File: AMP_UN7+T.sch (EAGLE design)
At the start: 55 parts

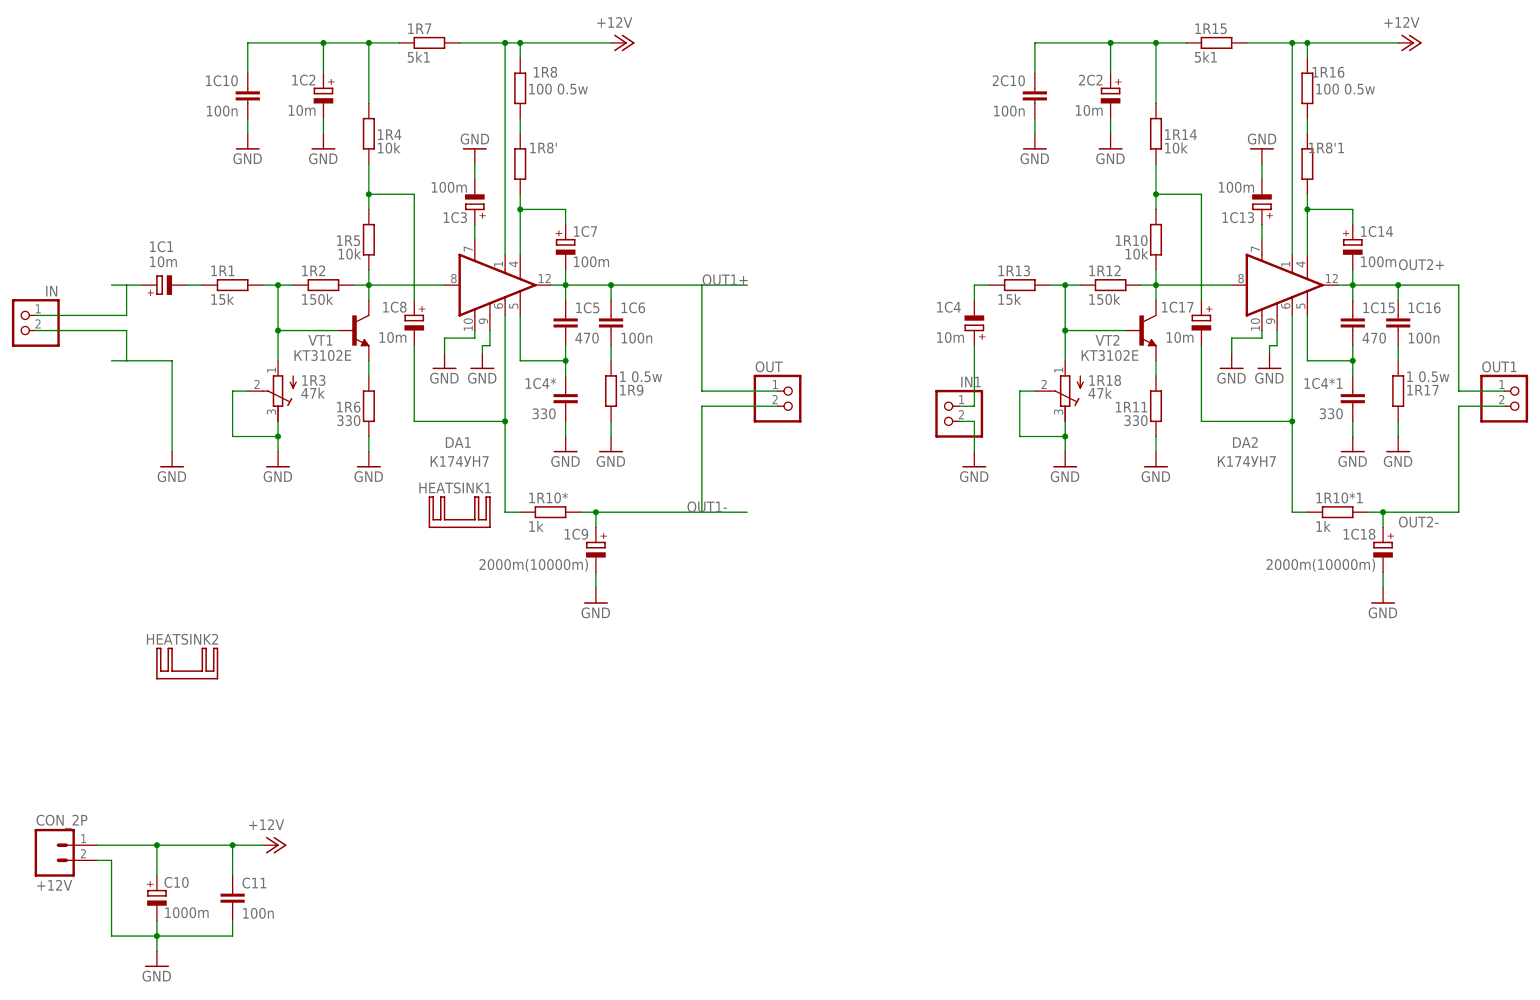
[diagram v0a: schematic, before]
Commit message: 4
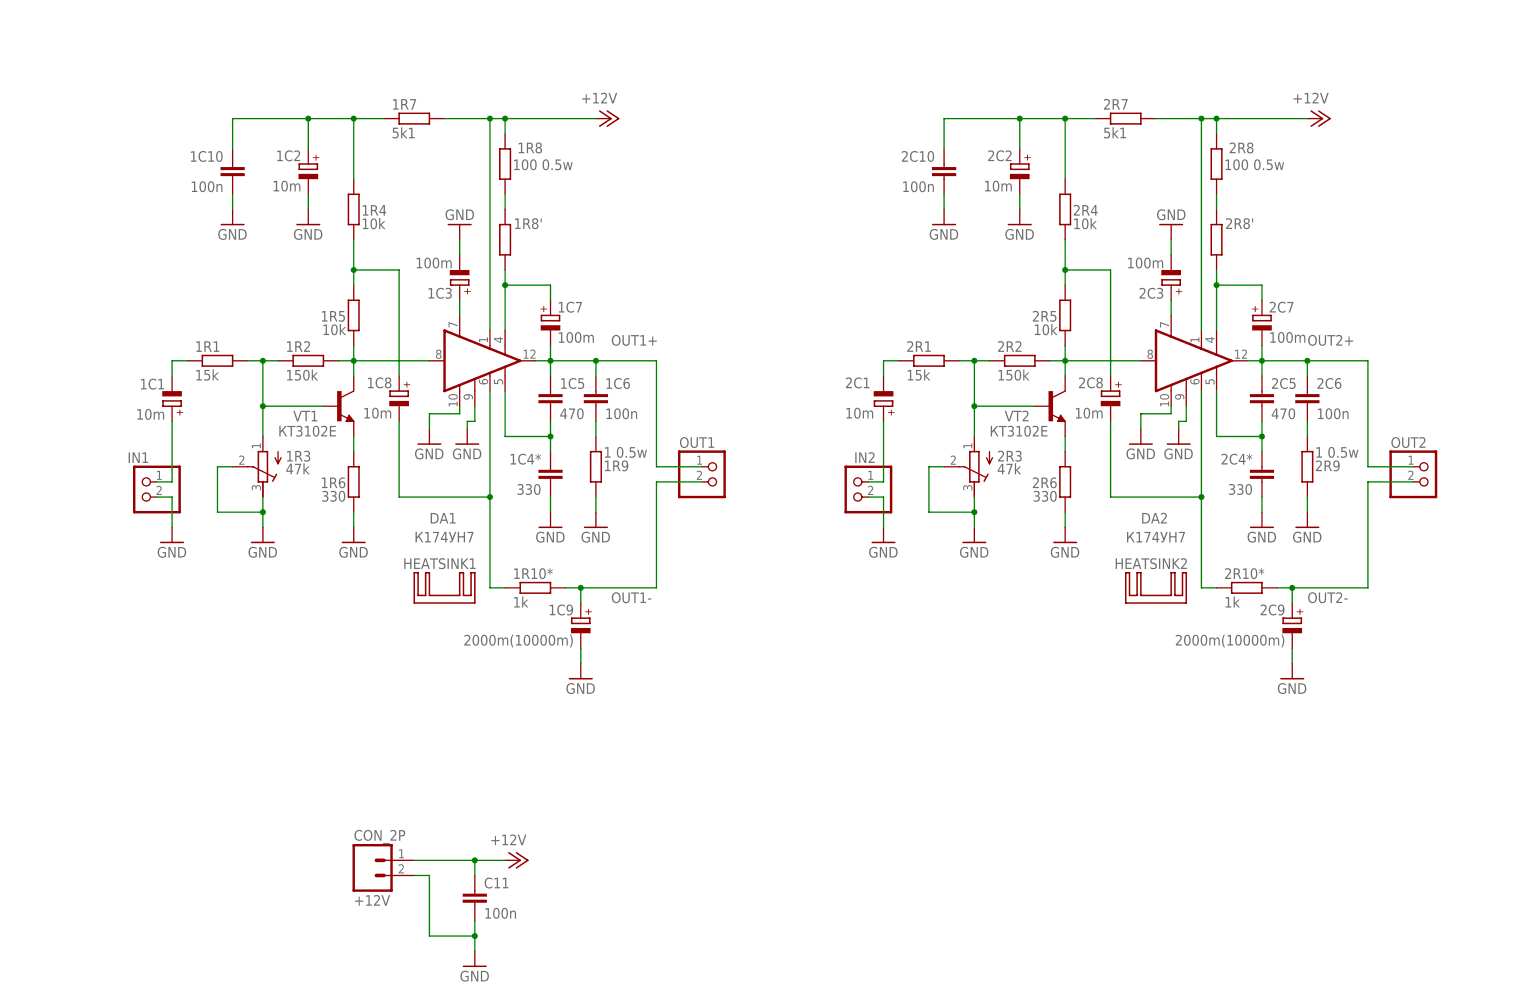
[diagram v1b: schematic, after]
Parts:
- removed 1C13: 100m, rcl:CPOL-EUE2.5-6
- removed 1C14: 100m, rcl:CPOL-EUE2.5-5
- removed 1C15: 470, rcl:C-EU050-030X075
- removed 1C16: 100n, rcl:C-EU075-052X106
- removed 1C17, 1C4: 10m, rcl:CPOL-EUE2.5-5
- removed 1C18: 2000m(10000m), rcl:CPOL-EUE5-13
- removed 1C4*1: 330, rcl:C-EU050-025X075
- removed 1R10, 1R14: 10k, rcl:R-EU_R0805
- removed 1R10*1: 1k, rcl:R-EU_0207/12
- removed 1R11: 330, rcl:R-EU_R0805
- removed 1R12: 150k, rcl:R-EU_R0805
- removed 1R13: 15k, rcl:R-EU_R0805
- removed 1R15: 5k1, rcl:R-EU_R0805
- removed 1R16: 100 0.5w, rcl:R-EU_R1210W
- removed 1R17: 1 0.5w, rcl:R-EU_0411/3V
- removed 1R18: 47k, rcl:R-TRIMM3296W
- removed 1R8'1: (no value), rcl:R-EU_R1210W
- removed C10: 1000m, rcl:CPOL-EUE5-13
- removed IN, OUT: (no value), pinhead:PINHD-1X2
- added 2C1, 2C8: 10m, rcl:CPOL-EUE2.5-5
- added 2C3: 100m, rcl:CPOL-EUE2.5-6
- added 2C4*: 330, rcl:C-EU050-025X075
- added 2C5: 470, rcl:C-EU050-030X075
- added 2C6: 100n, rcl:C-EU075-052X106
- added 2C7: 100m, rcl:CPOL-EUE2.5-5
- added 2C9: 2000m(10000m), rcl:CPOL-EUE5-13
- added 2R1: 15k, rcl:R-EU_R0805
- added 2R10*: 1k, rcl:R-EU_0207/12
- added 2R2: 150k, rcl:R-EU_R0805
- added 2R3: 47k, rcl:R-TRIMM3296W
- added 2R4, 2R5: 10k, rcl:R-EU_R0805
- added 2R6: 330, rcl:R-EU_R0805
- added 2R7: 5k1, rcl:R-EU_R0805
- added 2R8: 100 0.5w, rcl:R-EU_R1210W
- added 2R8': (no value), rcl:R-EU_R1210W
- added 2R9: 1 0.5w, rcl:R-EU_0411/3V
- added IN2, OUT2: (no value), pinhead:PINHD-1X2
- +12V: device DSS:CON_2P -> untitled:CON_2P
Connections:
- removed net N$27: 1C4.+, IN1.1
- removed net N$7: 1C1.+, IN.1
- new net IN1: 1C1.+, IN1.1
- new net IN2: 2C1.+, IN2.1
- net +12V: now also 2R7.2, 2R8.2; no longer 1R15.2, 1R16.2, C10.+
- net GND: now also 2C3.-, 2C4*.2, 2C9.-, 2R3.E, 2R3.S, 2R6.1, 2R9.2, IN2.2; no longer 1C13.-, 1C18.-, 1C4*1.2, 1R11.1, 1R17.2, 1R18.E, 1R18.S, C10.-, IN.2
- net N$16: now also 2R2.2, 2R5.1; no longer 1R10.1, 1R12.2
- net N$17: now also 2R6.2; no longer 1R11.2
- net N$18: now also 2R1.2, 2R2.1, 2R3.A; no longer 1R12.1, 1R13.2, 1R18.A
- net N$19: now also 2C1.-, 2R1.1; no longer 1C4.-, 1R13.1
- net N$20: now also 2C8.+, 2R4.1, 2R5.2; no longer 1C17.+, 1R10.2, 1R14.1
- net N$21: now also 2R4.2, 2R7.1; no longer 1R14.2, 1R15.1
- net N$22: now also 2C3.+; no longer 1C13.+
- net N$23: now also 2C7.+, 2R8'.1; no longer 1C14.+, 1R8'1.1
- net N$24: now also 2C4*.1, 2C5.2; no longer 1C15.2, 1C4*1.1
- net N$25: now also 2C6.2, 2R9.1; no longer 1C16.2, 1R17.1
- net N$26: now also 2C8.-, 2R10*.1; no longer 1C17.-, 1R10*1.1
- net N$28: now also 2R8'.2, 2R8.1; no longer 1R16.1, 1R8'1.2
- net OUT1+: now also OUT1.1; no longer OUT.1
- net OUT1-: now also OUT1.2; no longer OUT.2
- net OUT2+: now also 2C5.1, 2C6.1, 2C7.-, OUT2.1; no longer 1C14.-, 1C15.1, 1C16.1, OUT1.1
- net OUT2-: now also 2C9.+, 2R10*.2, OUT2.2; no longer 1C18.+, 1R10*1.2, OUT1.2
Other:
- note added: "УМЗЧ с малыми искажениями на ИС К174УН7"
- moved on the sheet: +12V, 1C1, 1C10, 1C2, 1C3, 1C4*, 1C5, 1C6, 1C7, 1C8, 1C9, 1R1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
